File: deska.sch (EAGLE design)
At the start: 18 parts, among them Q1 BC547, Q2 BC547

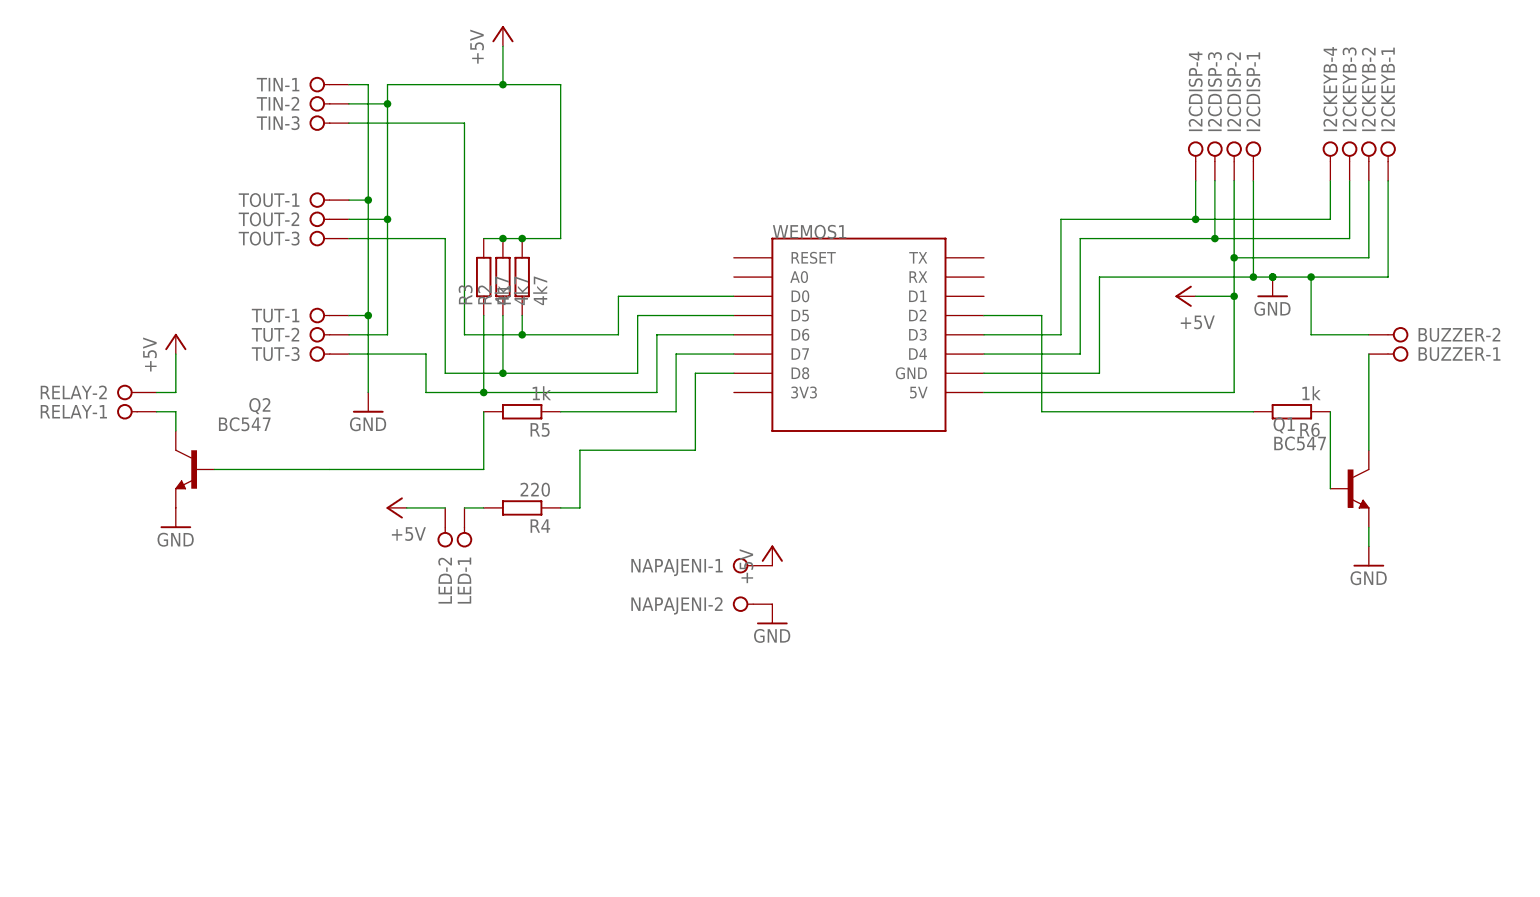
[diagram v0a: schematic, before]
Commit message: upravy desky
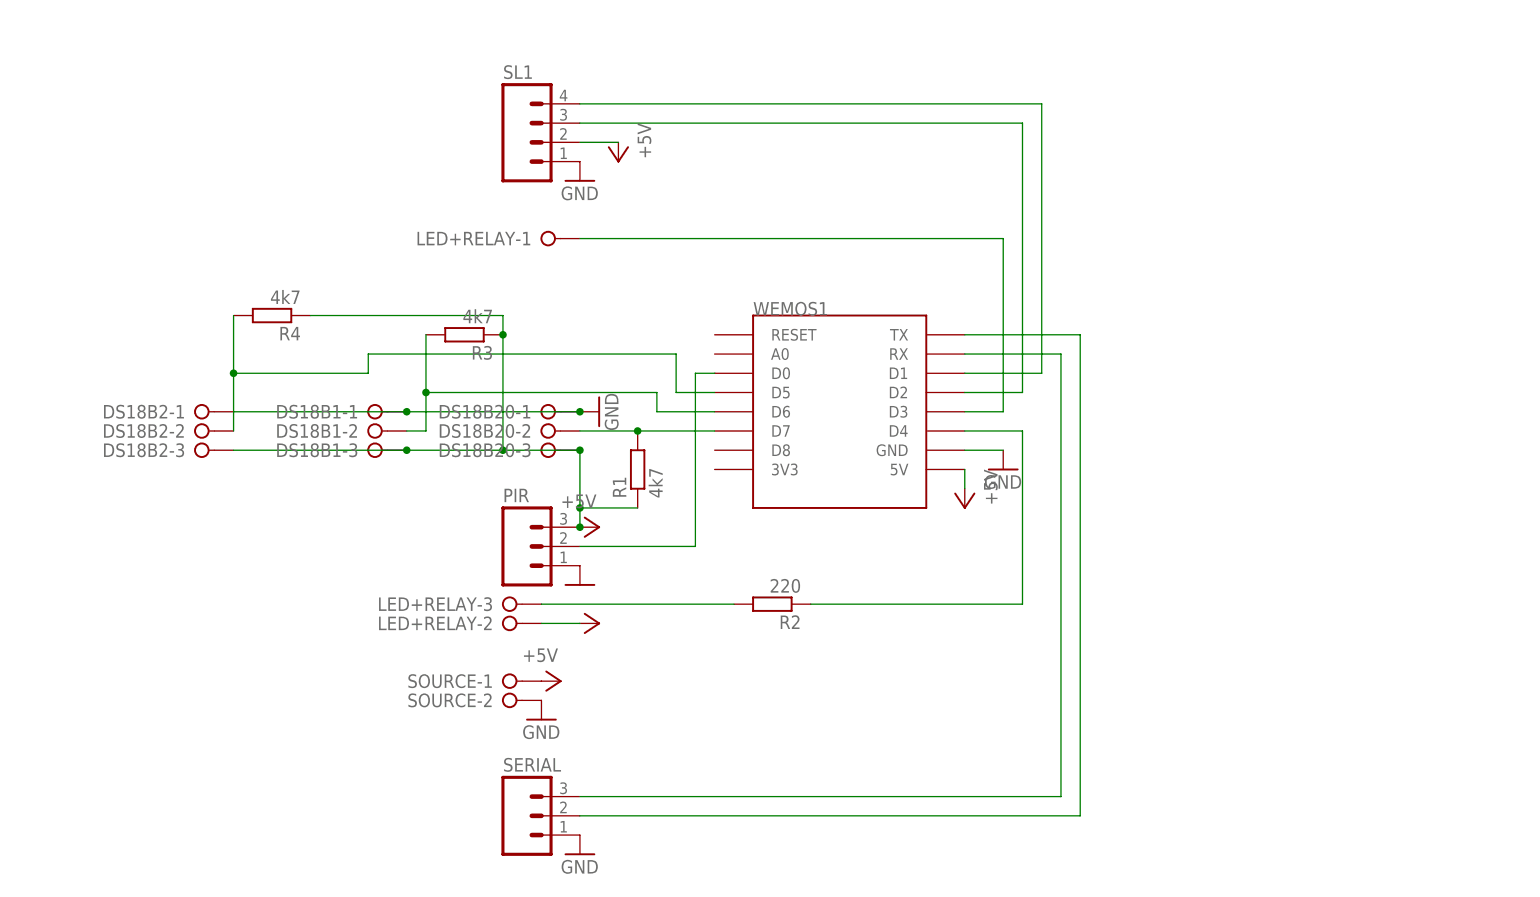
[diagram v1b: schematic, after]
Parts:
- removed BUZZER, LED, NAPAJENI, RELAY: (no value), con-wago-508:W237-02P
- removed I2CDISP, I2CKEYB: (no value), con-wago-508:W237-04P
- removed Q1, Q2: BC547, transistor-npn:BC547
- removed R5, R6: 1k, rcl:R-EU_0207/7
- removed TIN, TOUT, TUT: (no value), con-wago-508:W237-3E
- added DS18B1, DS18B2, DS18B20, LED+RELAY: (no value), con-wago-508:W237-03P
- added PIR, SERIAL: (no value), con-amp-quick:M03
- added SL1: (no value), con-amp-quick:M04
- added SOURCE: (no value), con-wago-508:W237-02P
- R1, R3: device rcl:R-EU_0207/7 -> rcl:R-EU_0207/10
- R2: value 4k7 -> 220; device rcl:R-EU_0207/7 -> rcl:R-EU_0207/10
- R4: value 220 -> 4k7; device rcl:R-EU_0207/7 -> rcl:R-EU_0207/10
- WEMOS1: device wemos:WEMOS-D1-MINI -> esp8266modules:WEMOS-D1-MINI
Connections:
- removed net N$12: I2CDISP-3.KL, I2CKEYB-3.KL, WEMOS1.D4
- removed net N$14: Q2.C, RELAY-1.KL
- removed net N$15: BUZZER-1.KL, Q1.C
- removed net N$16: R6.2, WEMOS1.D2
- removed net N$19: R2.1, TOUT-3.KL, WEMOS1.D5
- new net N$2: SERIAL.3, WEMOS1.RX
- new net N$8: LED+RELAY-3.KL, R2.2
- new net N$9: DS18B20-2.KL, R1.2, WEMOS1.D7
- net +5V: now also DS18B1-3.KL, DS18B2-3.KL, DS18B20-3.KL, LED+RELAY-2.KL, PIR.3, R1.1, R3.1, R4.1, SL1.2, SOURCE-1.KL; no longer I2CDISP-2.KL, I2CKEYB-2.KL, LED-2.KL, NAPAJENI-1.KL, R1.2, R2.2, R3.2, RELAY-2.KL, TIN-2.KL, TOUT-2.KL, TUT-2.KL
- net GND: now also DS18B1-1.KL, DS18B2-1.KL, DS18B20-1.KL, PIR.1, SERIAL.1, SL1.1, SOURCE-2.KL; no longer BUZZER-2.KL, I2CDISP-1.KL, I2CKEYB-1.KL, NAPAJENI-2.KL, Q1.E, Q2.E, TIN-1.KL, TOUT-1.KL, TUT-1.KL
- net N$1: now also SERIAL.2, WEMOS1.TX; no longer R1.1, TIN-3.KL, WEMOS1.D0
- net N$11: now also DS18B2-2.KL, R4.2, WEMOS1.D5; no longer I2CDISP-4.KL, I2CKEYB-4.KL, WEMOS1.D3
- net N$13: now also DS18B1-2.KL, R3.2, WEMOS1.D6; no longer Q2.B, R5.2
- net N$3: now also SL1.4, WEMOS1.D1; no longer R3.1, TUT-3.KL, WEMOS1.D6
- net N$4: now also SL1.3, WEMOS1.D2; no longer R5.1, WEMOS1.D7
- net N$5: now also PIR.2, WEMOS1.D0; no longer R4.1, WEMOS1.D8
- net N$6: now also R2.1, WEMOS1.D4; no longer LED-1.KL, R4.2
- net N$7: now also LED+RELAY-1.KL, WEMOS1.D3; no longer Q1.B, R6.1
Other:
- moved on the sheet: R1, R2, R3, R4, WEMOS1
